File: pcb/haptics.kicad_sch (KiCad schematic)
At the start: 14 parts, among them J7 1751248, J8 1751248, U1 DRV2605LDGS, U3 DRV2605LDGS

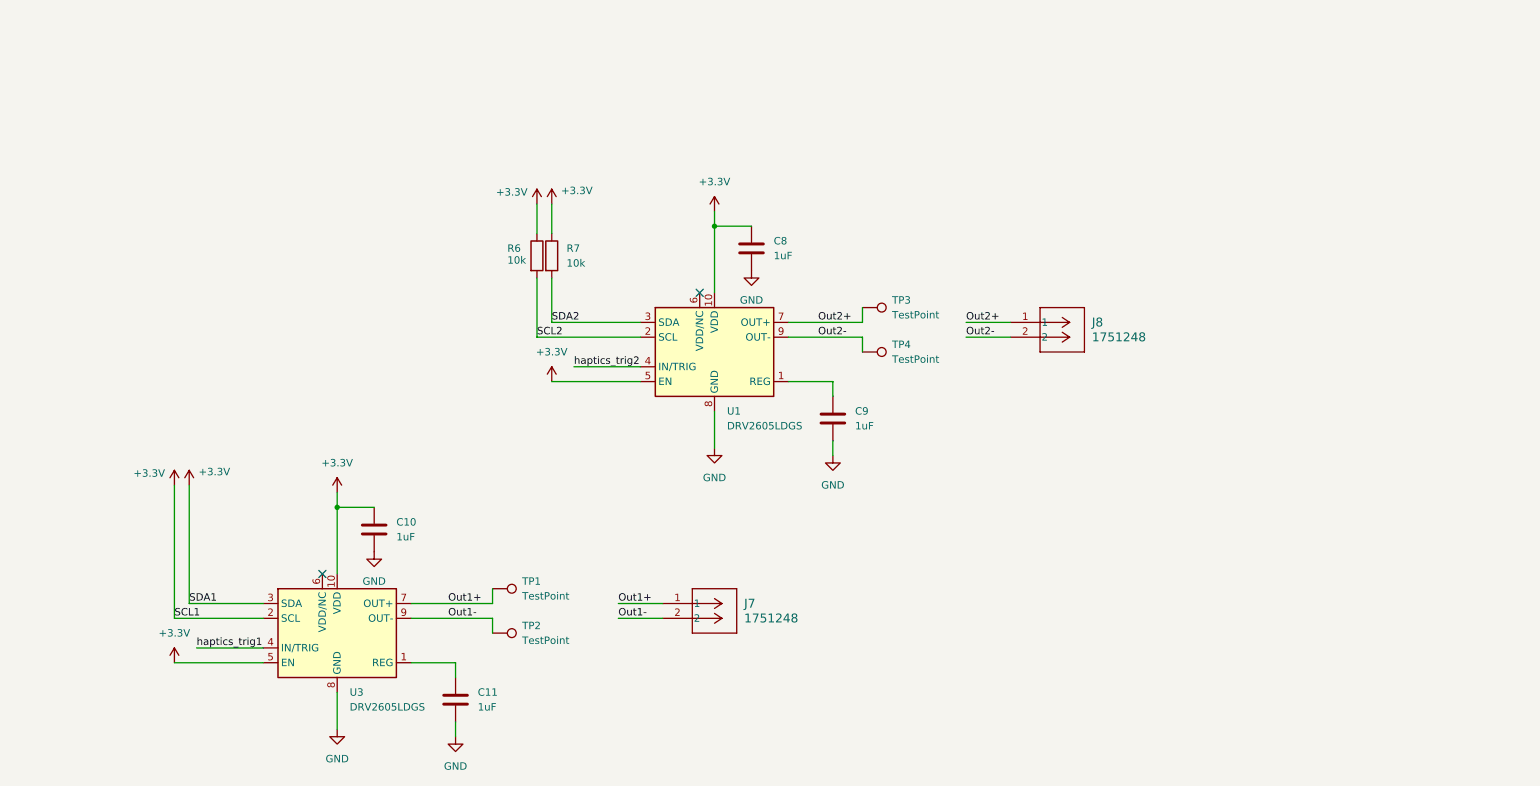
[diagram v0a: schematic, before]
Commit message: stuff
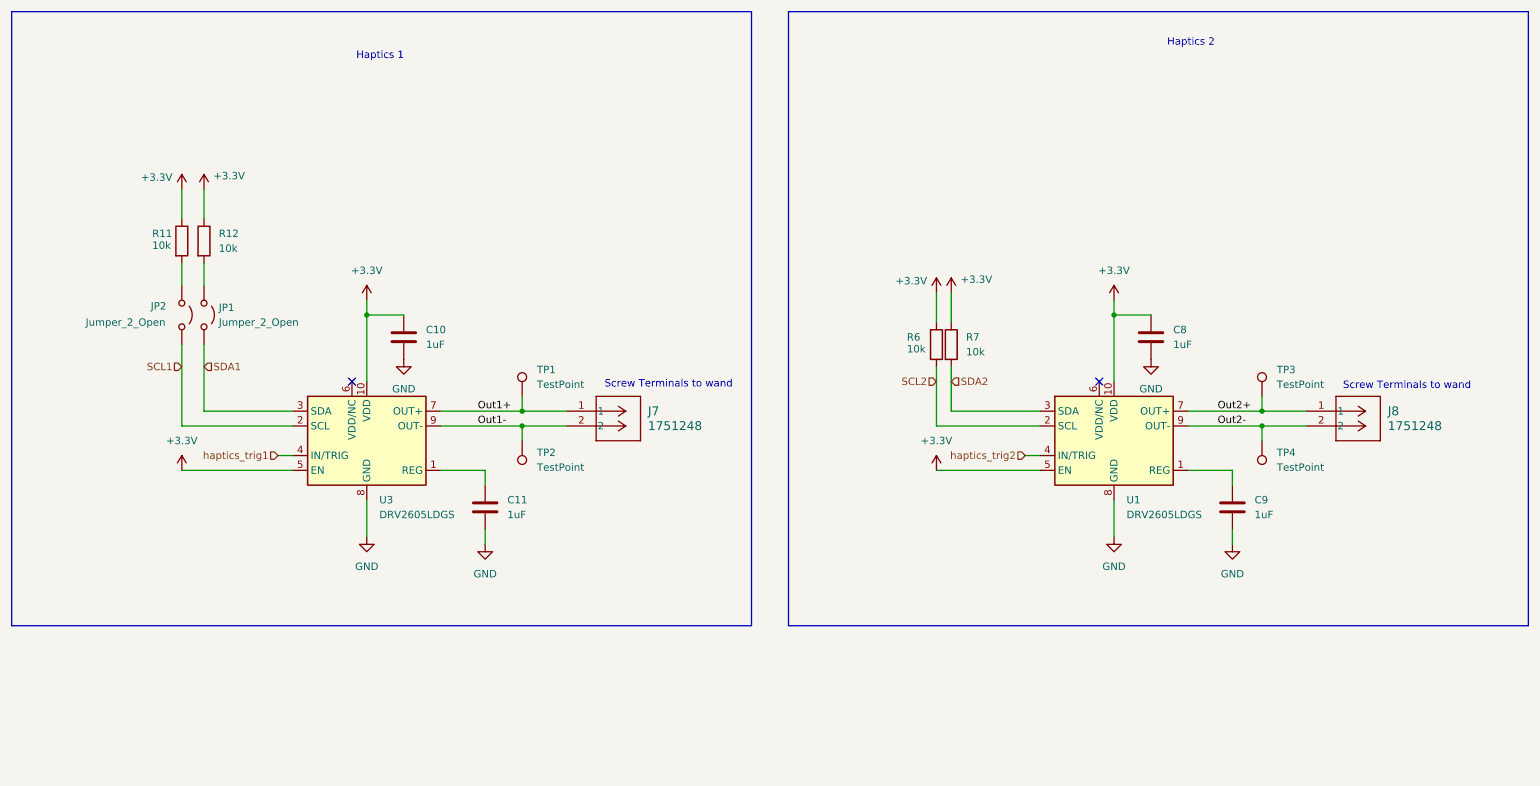
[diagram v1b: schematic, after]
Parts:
- added JP1, JP2: Jumper_2_Open, TestPoint:TestPoint_2Pads_Pitch2.54mm_Drill0.8mm, symbol Jumper:Jumper_2_Open
- added R11, R12: 10k, Resistor_SMD:R_0603_1608Metric, symbol Device:R
- C10, C11, C8, C9: footprint (none) -> Capacitor_SMD:C_0603_1608Metric
- J7, J8: footprint CONN_1751248_PXC -> 2x1term:CONN_1751248_PXC
- R6, R7: footprint (none) -> Resistor_SMD:R_0603_1608Metric
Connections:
- net +3.3V: now also R11.1, R12.1; no longer U3.2 (SCL), U3.3 (SDA)
- new net: JP1.1 (A), R12.2
- new net: JP2.1 (A), R11.2
- new net SCL1: JP2.2 (B), U3.2 (SCL)
- new net SDA1: JP1.2 (B), U3.3 (SDA)
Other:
- note added: "Haptics 1"
- note added: "Haptics 2"
- note added: "Screw Terminals to wand"
- moved on the sheet: C10, C11, C8, C9, J7, J8, R6, R7, TP1, TP2, TP3, TP4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
